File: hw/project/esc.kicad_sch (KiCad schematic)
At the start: 0 parts

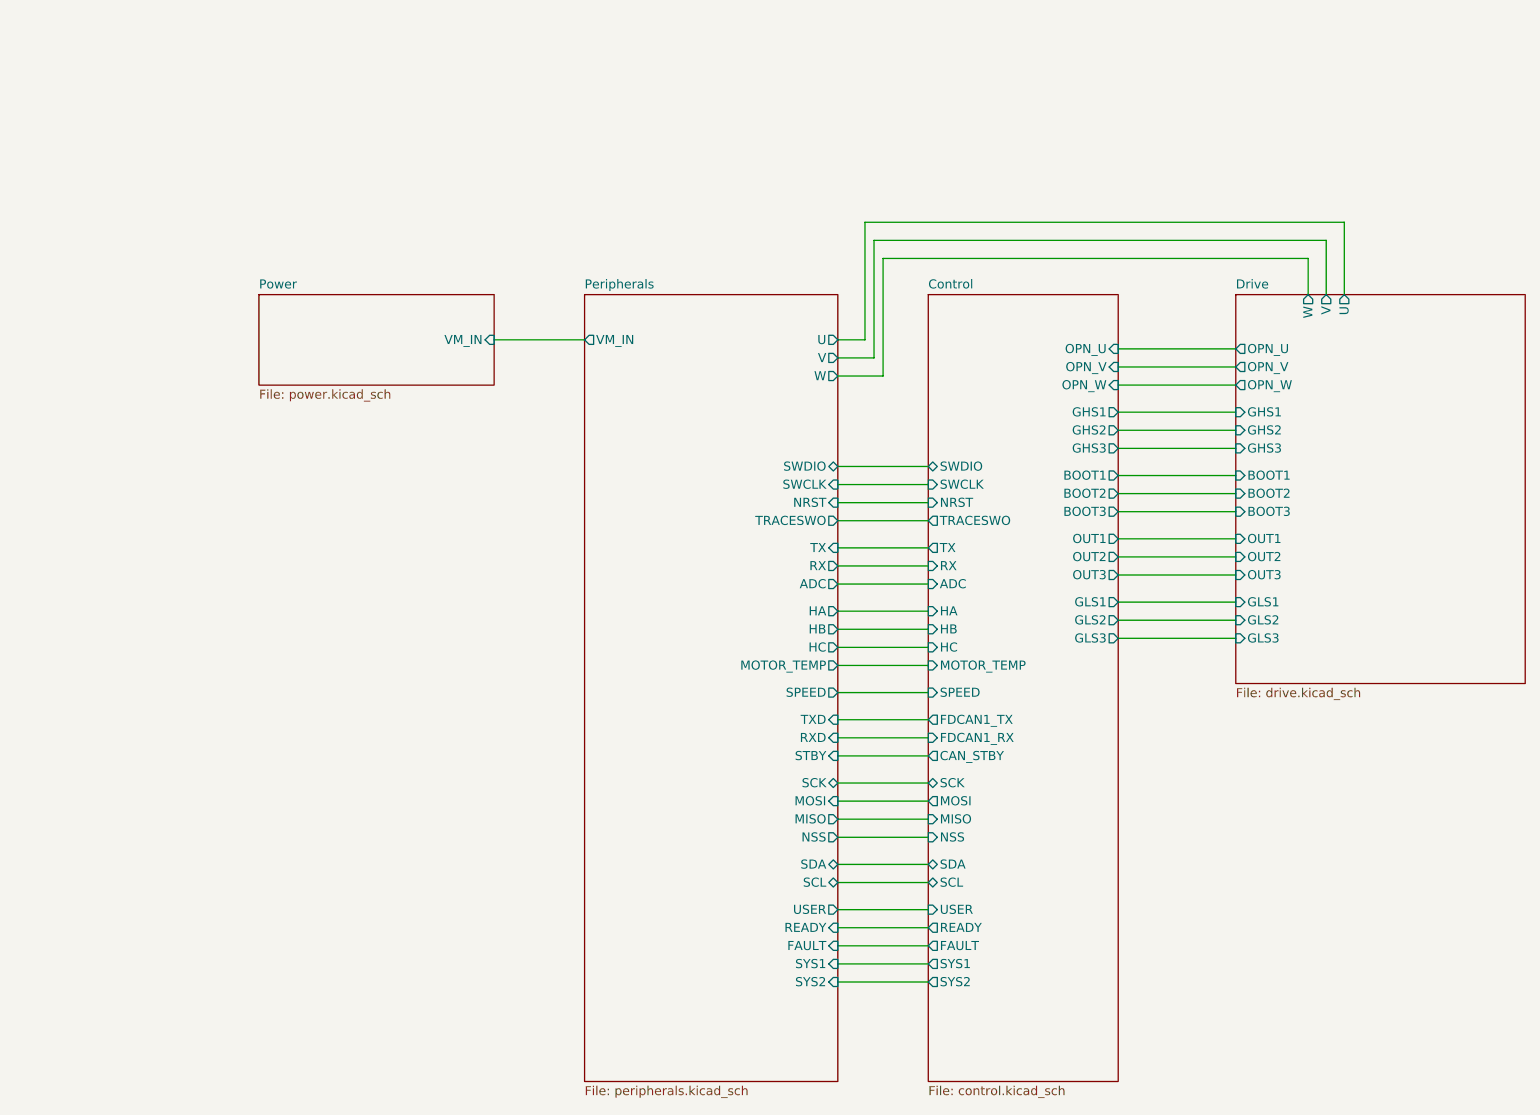
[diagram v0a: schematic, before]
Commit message: stm header and minor changes
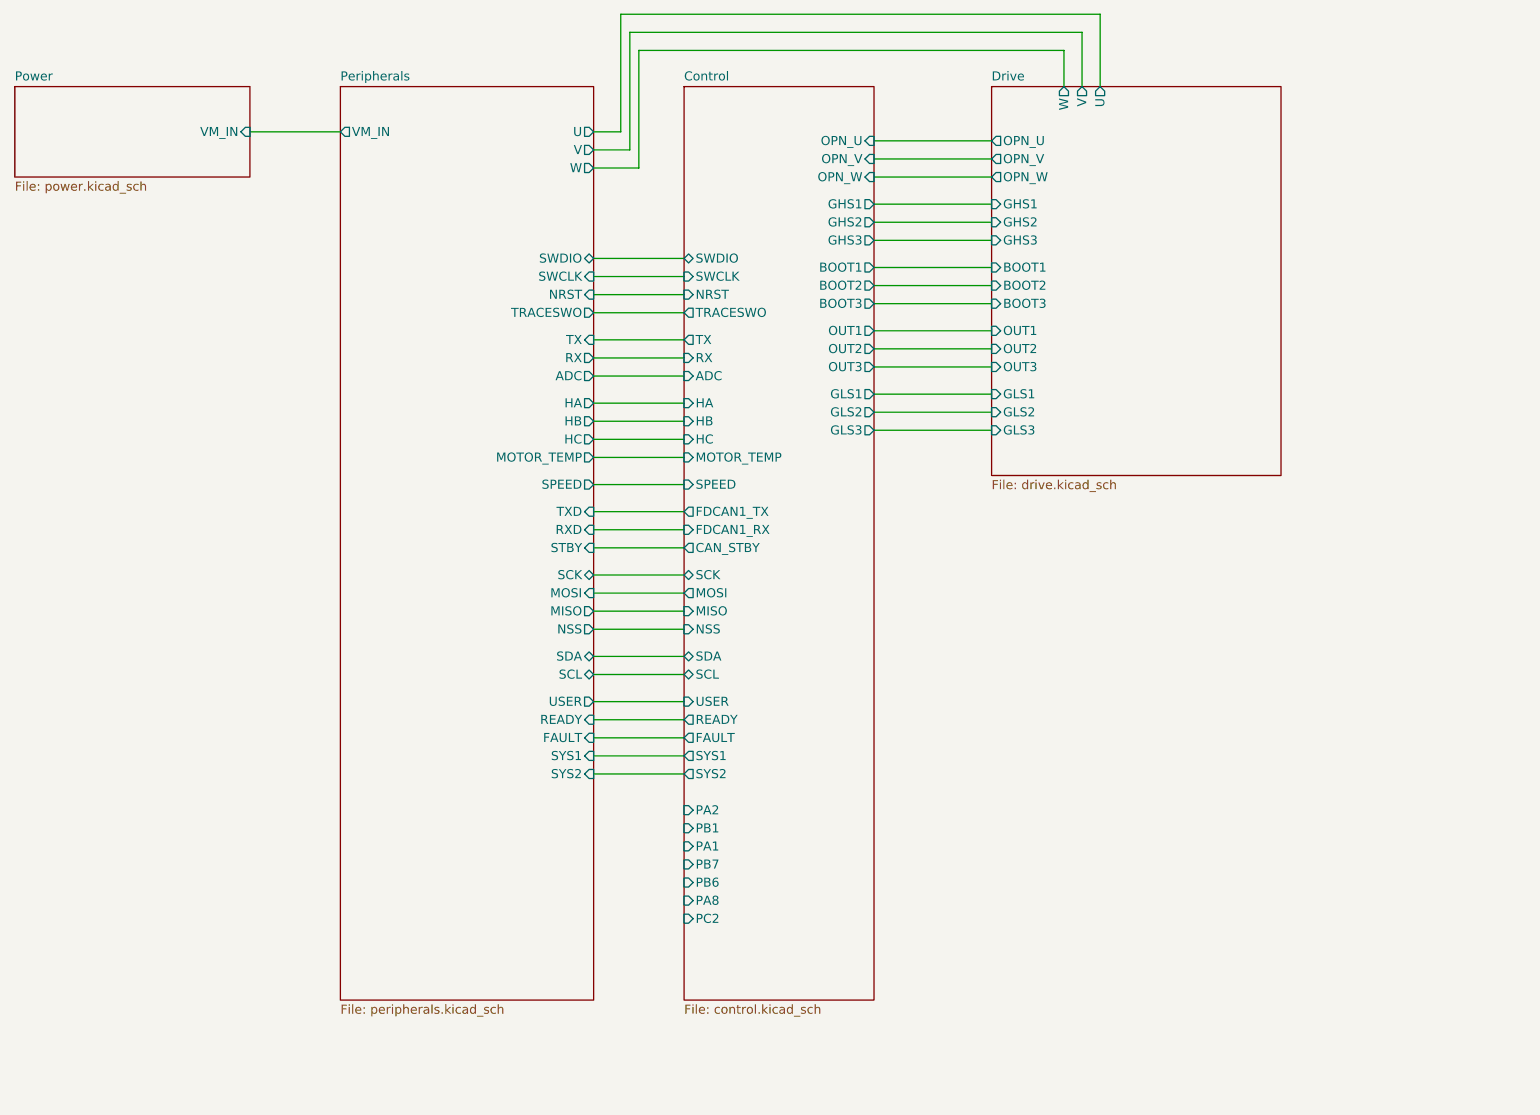
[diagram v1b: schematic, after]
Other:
- sheet Control ports: added PA1, PA2, PA8, PB1, PB6, PB7, PC2; removed none
